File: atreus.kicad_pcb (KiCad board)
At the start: 2 copper layers, 232 x 90 mm, 85 parts

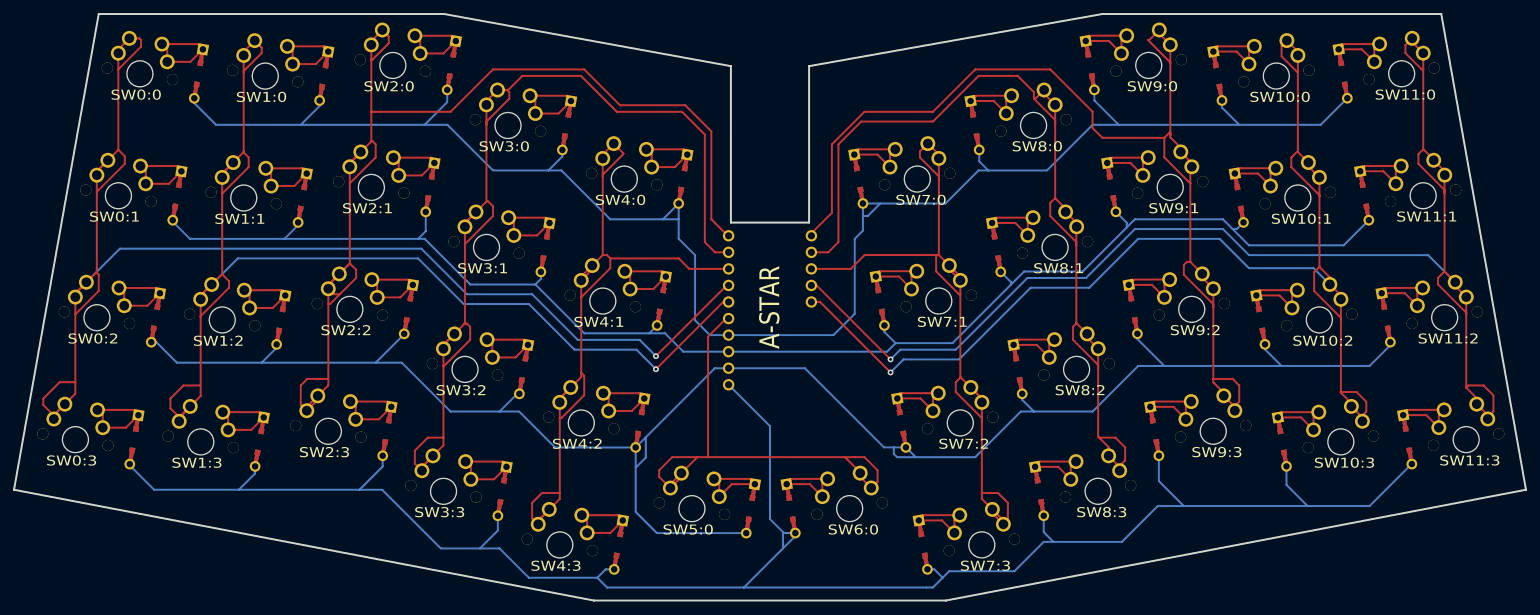
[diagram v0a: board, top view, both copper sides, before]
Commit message: Generate up to date kicad_pcb file
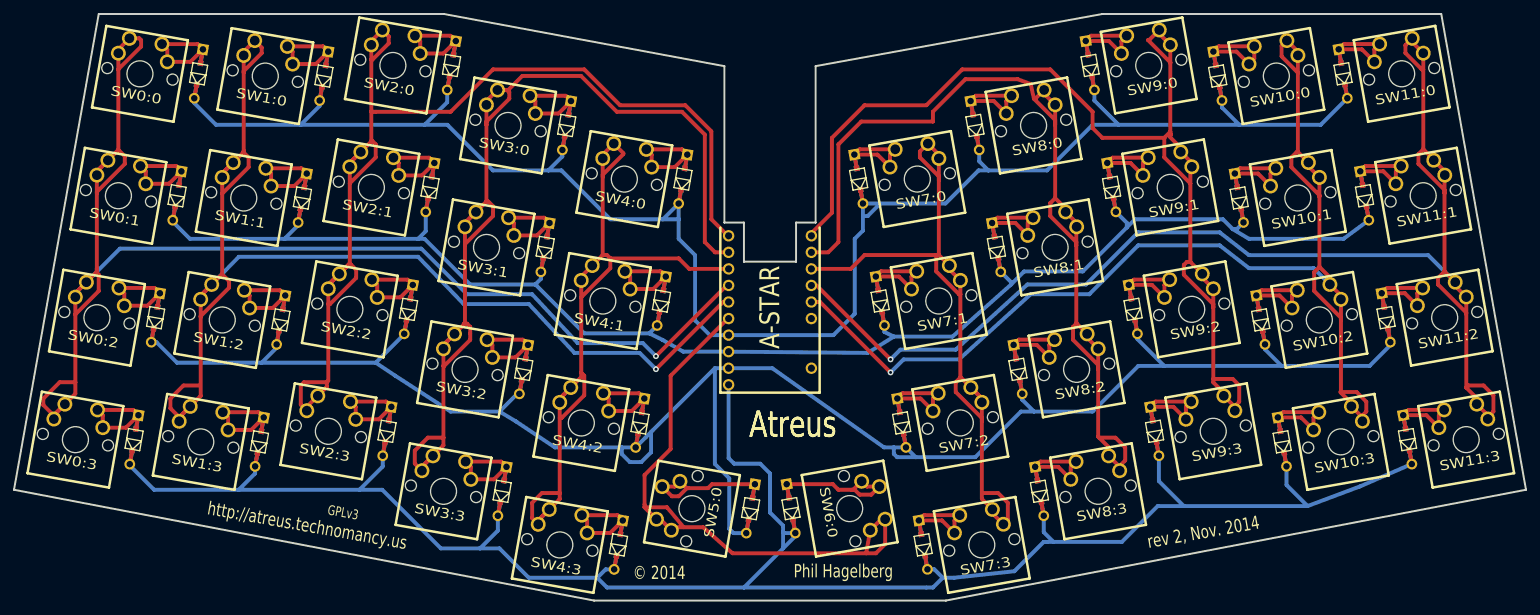
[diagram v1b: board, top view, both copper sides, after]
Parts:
- turned SW5:0 to 80 degrees
- turned SW6:0 to 280 degrees
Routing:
- net N-col-5: track 80.4 -> 92.9 mm
- net N-col-2: track 189.2 -> 183.7 mm
- net N-col-6: track 124.5 -> 119.2 mm
- net N-diode-20: track 15.9 -> 20.4 mm
- net N-diode-24: track 15.9 -> 20.3 mm
- net N-row-0: track 264.8 -> 261.4 mm
- net (no net): track 0.00 -> 3.46 mm
- net N-row-1: track 226.9 -> 223.8 mm
- net N-col-4: track 124.1 -> 121.2 mm
- net N-row-2: track 281.8 -> 283.8 mm
- net N-col-9: track 193.0 -> 191.6 mm
- net N-col-10: track 211.5 -> 210.6 mm
- net N-col-8: track 176.2 -> 176.8 mm
- net N-col-7: track 153.6 -> 154.2 mm
- net N-row-3: track 299.5 -> 300.1 mm
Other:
- outline, holes or cut-outs redrawn
- board text added: "Atreus"
- board text added: "GPLv3"
- board text added: "Phil Hagelberg"
- board text added: "http://atreus.technomancy.us"
- board text added: "rev 2, Nov. 2014"
- board text added: "© 2014"

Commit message: Remove linear net numbering hack
Works with KiCad 5.1.4 and it it also makes it easier to further extend the PCB
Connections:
- net N-diode-21 renamed N-diode-42
- net N-diode-22 renamed N-diode-43
- net N-diode-23 renamed N-diode-44
- net N-diode-25 renamed N-diode-45
- net N-diode-26 renamed N-diode-46
- net N-diode-27 renamed N-diode-47
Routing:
- net N-diode-42: track 15.9 -> 0.00 mm
- net N-diode-21: track 0.00 -> 15.9 mm
- net N-diode-45: track 15.9 -> 0.00 mm
- net N-diode-25: track 0.00 -> 15.9 mm
- net N-diode-46: track 15.9 -> 0.00 mm
- net N-diode-26: track 0.00 -> 15.9 mm
- net N-diode-47: track 15.9 -> 0.00 mm
- net N-diode-43: track 15.9 -> 0.00 mm
- net N-diode-27: track 0.00 -> 15.9 mm
- net N-diode-22: track 0.00 -> 15.9 mm
- net N-diode-44: track 15.9 -> 0.00 mm
- net N-diode-23: track 0.00 -> 15.9 mm
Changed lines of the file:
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@@
 (net 56 N-diode-40)
 (net 57 N-diode-41)
+(net 58 N-diode-42)
+(net 59 N-diode-43)
+(net 60 N-diode-44)
+(net 61 N-diode-45)
+(net 62 N-diode-46)
+(net 63 N-diode-47)
 (net_class
  Default
@@
  (add_net N-diode-39)
  (add_net N-diode-40)
- (add_net N-diode-41))
+ (add_net N-diode-41)
+ (add_net N-diode-42)
+ (add_net N-diode-43)
+ (add_net N-diode-44)
+ (add_net N-diode-45)
+ (add_net N-diode-46)
+ (add_net N-diode-47))
 (module A_STAR (layer Front)
   (at 134 70 270)
@@
    (drill 1.4986)
    (layers *.Cu *.SilkS *.Mask)
-   (net 37 N-diode-21))
+   (net 58 N-diode-42))
   (pad
    2
@@
    (drill 1.4986)
    (layers *.Cu *.SilkS *.Mask)
-   (net 37 N-diode-21)))
+   (net 58 N-diode-42)))
 (module DIODE (layer Front)
   (at 209.2916920192295 68.9392642471365 100)
@@
    (drill 0.9906)
    (layers *.Cu *.SilkS *.Mask)
-   (net 37 N-diode-21))
+   (net 58 N-diode-42))
   (pad
    99
@@
    (drill 1.4986)
    (layers *.Cu *.SilkS *.Mask)
-   (net 38 N-diode-22))
+   (net 59 N-diode-43))
   (pad
    2
@@
    (drill 1.4986)
    (layers *.Cu *.SilkS *.Mask)
-   (net 38 N-diode-22)))
+   (net 59 N-diode-43)))
 (module DIODE (layer Front)
   (at 212.59100739490117 87.65061155436845 100)
@@
    (drill 0.9906)
    (layers *.Cu *.SilkS *.Mask)
-   (net 38 N-diode-22))
+   (net 59 N-diode-43))
   (pad
    99
@@
    (drill 1.4986)
    (layers *.Cu *.SilkS *.Mask)
-   (net 39 N-diode-23))
+   (net 60 N-diode-44))
   (pad
    2
@@
    (drill 1.4986)
    (layers *.Cu *.SilkS *.Mask)
-   (net 39 N-diode-23)))
+   (net 60 N-diode-44)))
 (module DIODE (layer Front)
   (at 221.92535310811888 31.171677516037544 100)
@@
    (drill 0.9906)
    (layers *.Cu *.SilkS *.Mask)
-   (net 39 N-diode-23))
+   (net 60 N-diode-44))
   (pad
    99
@@
    (drill 1.4986)
    (layers *.Cu *.SilkS *.Mask)
-   (net 41 N-diode-25))
+   (net 61 N-diode-45))
   (pad
    2
@@
    (drill 1.4986)
    (layers *.Cu *.SilkS *.Mask)
-   (net 41 N-diode-25)))
+   (net 61 N-diode-45)))
 (module DIODE (layer Front)
   (at 225.22466848379057 49.883024823269494 100)
@@
    (drill 0.9906)
    (layers *.Cu *.SilkS *.Mask)
-   (net 41 N-diode-25))
+   (net 61 N-diode-45))
   (pad
    99
@@
    (drill 1.4986)
    (layers *.Cu *.SilkS *.Mask)
-   (net 42 N-diode-26))
+   (net 62 N-diode-46))
   (pad
    2
@@
    (drill 1.4986)
    (layers *.Cu *.SilkS *.Mask)
-   (net 42 N-diode-26)))
+   (net 62 N-diode-46)))
 (module DIODE (layer Front)
   (at 228.52398385946222 68.59437213050145 100)
@@
    (drill 0.9906)
    (layers *.Cu *.SilkS *.Mask)
-   (net 42 N-diode-26))
+   (net 62 N-diode-46))
   (pad
    99
@@
    (drill 1.4986)
    (layers *.Cu *.SilkS *.Mask)
-   (net 43 N-diode-27))
+   (net 63 N-diode-47))
   (pad
    2
@@
    (drill 1.4986)
    (layers *.Cu *.SilkS *.Mask)
-   (net 43 N-diode-27)))
+   (net 63 N-diode-47)))
 (module DIODE (layer Front)
   (at 231.8232992351339 87.3057194377334 100)
@@
    (drill 0.9906)
    (layers *.Cu *.SilkS *.Mask)
-   (net 43 N-diode-27))
+   (net 63 N-diode-47))
   (pad
    99
